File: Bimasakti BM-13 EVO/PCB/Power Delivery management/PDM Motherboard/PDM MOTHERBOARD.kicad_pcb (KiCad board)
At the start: 2 copper layers, 77 x 73.1 mm, 43 parts

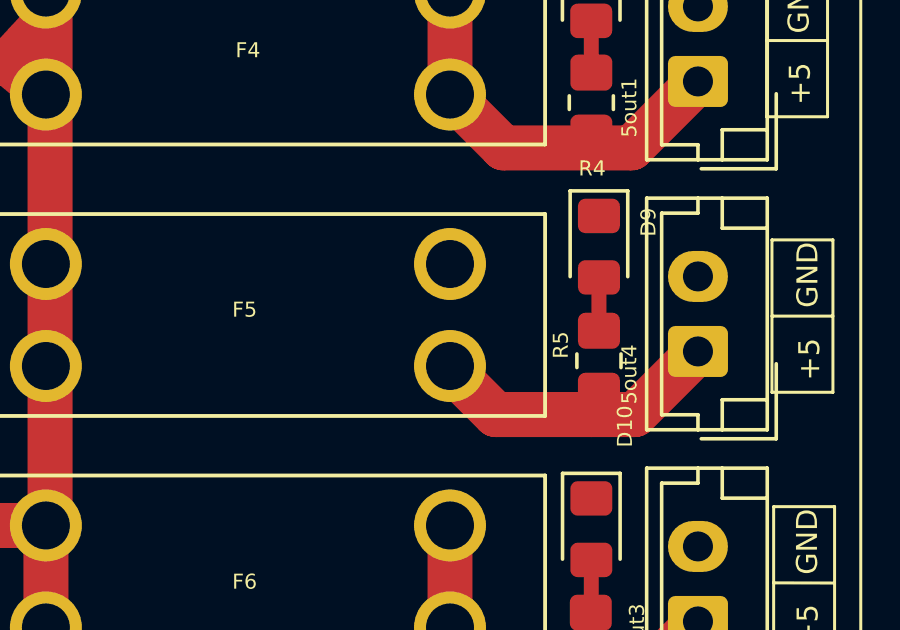
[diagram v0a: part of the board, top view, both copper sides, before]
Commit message: pdm and tv fix
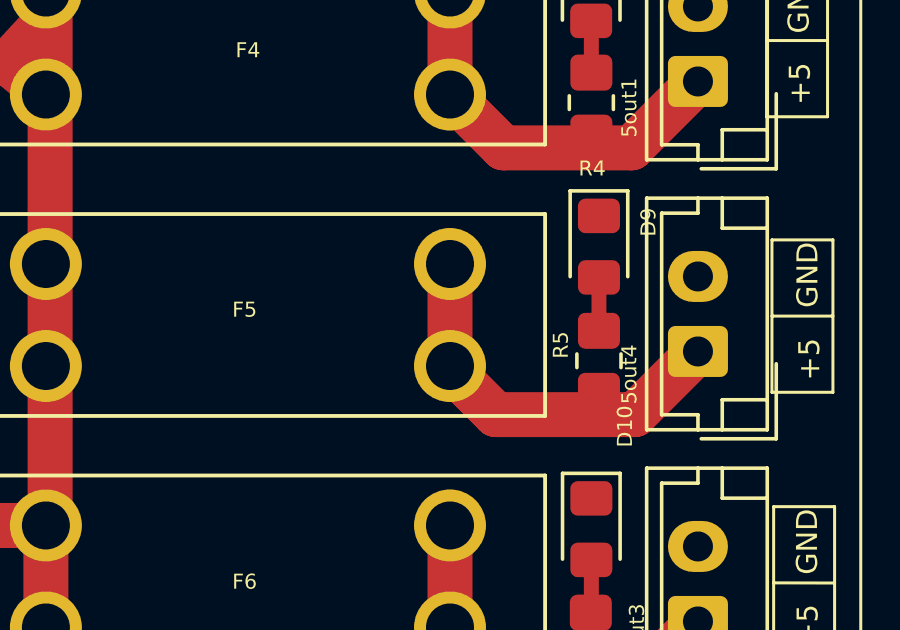
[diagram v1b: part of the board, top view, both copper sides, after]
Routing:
- net Net-(5out4-Pin_1): track 9.77 -> 13.2 mm
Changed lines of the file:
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@@
+	)
+	(segment
+		(start 134.735 65.084753)
+		(end 134.735 68.484753)
+		(width 1.5)
+		(layer "F.Cu")
+		(net 7)
 	)
 	(segment
